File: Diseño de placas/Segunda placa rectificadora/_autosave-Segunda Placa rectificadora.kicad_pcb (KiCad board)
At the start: 2 copper layers, 60 x 70 mm, 9 parts, among them J1 Screw_Terminal_01x02, J2 Screw_Terminal_01x02, J3 Screw_Terminal_01x02, J4 Screw_Terminal_01x02, J9 Screw_Terminal_01x02

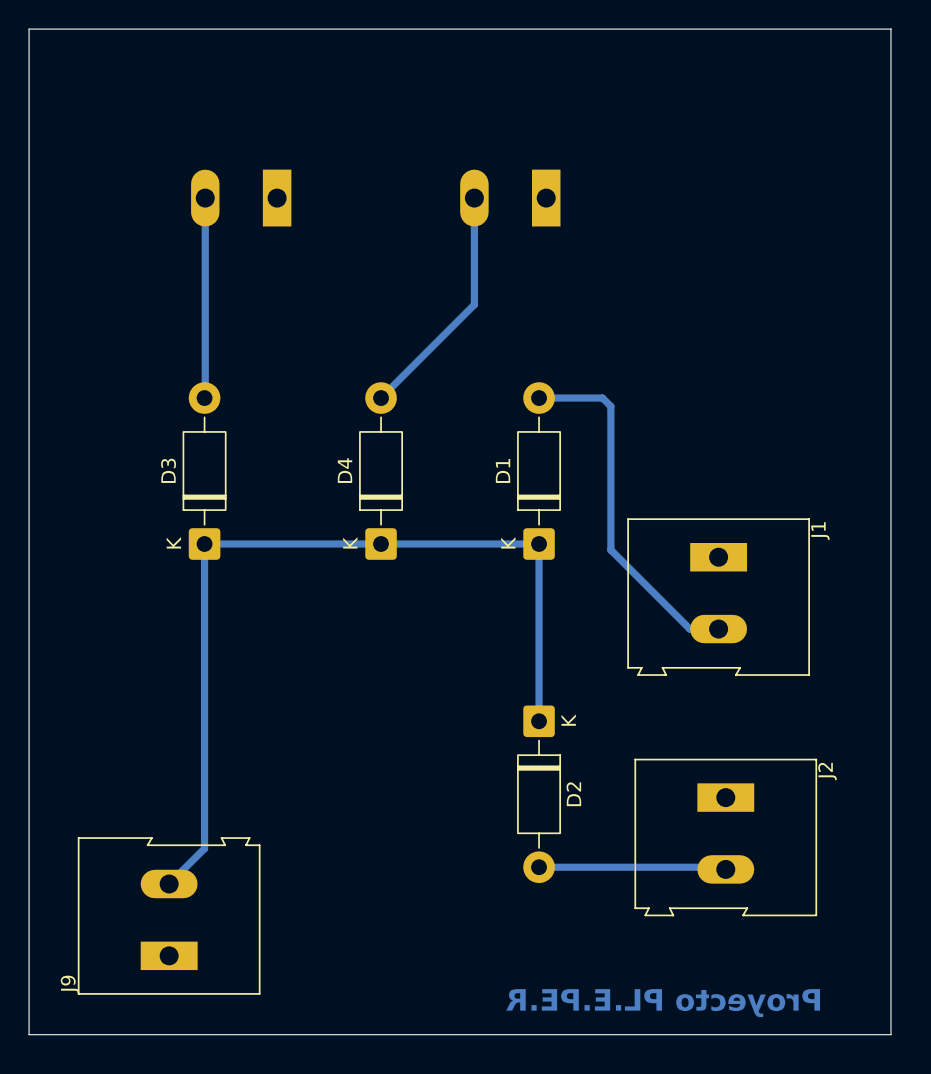
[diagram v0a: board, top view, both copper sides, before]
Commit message: Subo fotos grupales
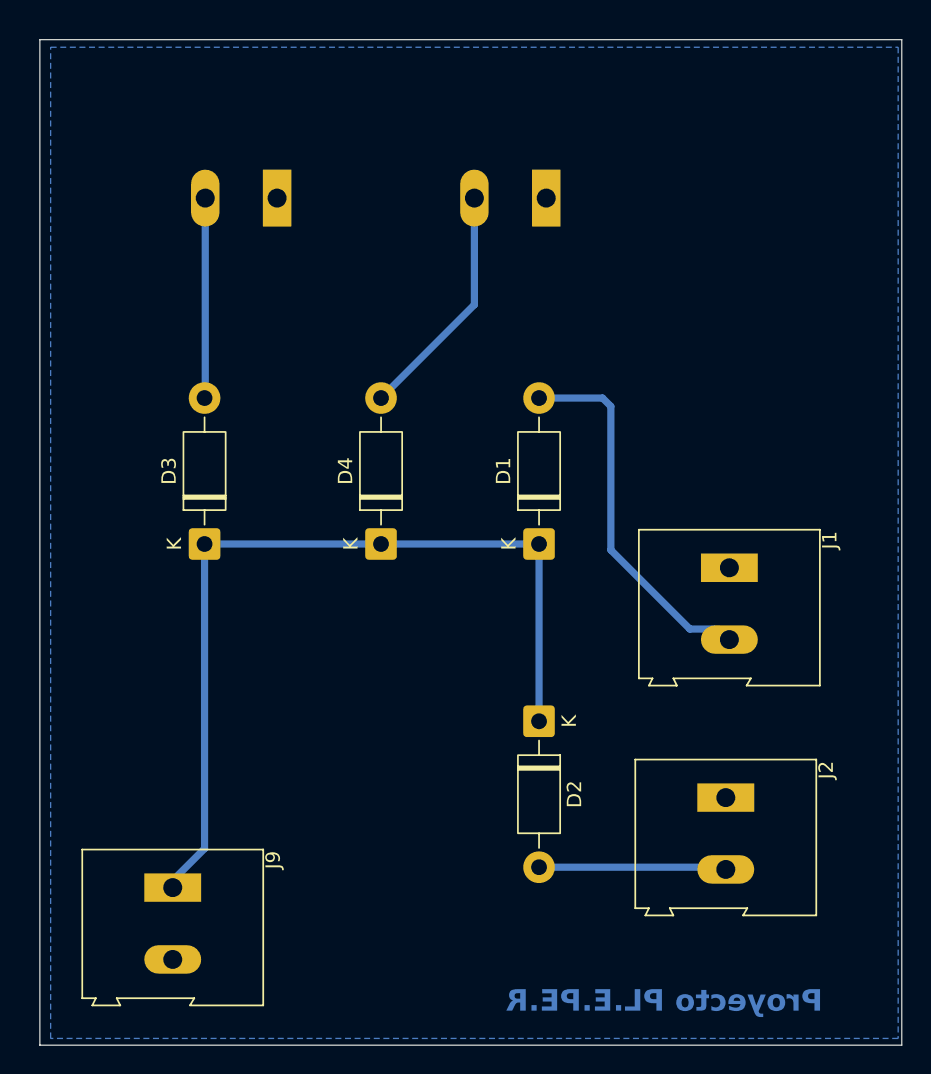
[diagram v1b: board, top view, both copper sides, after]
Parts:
- moved J9 4.76 mm to (94.5, 128.5), turned to -90 degrees
- moved J1 1.05 mm to (133.2, 106.2)
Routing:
- added copper zone on B.Cu, net Earth
